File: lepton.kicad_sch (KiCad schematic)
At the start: 33 parts, among them U10 ME6216A28XG, U12 3N25000G33YC, U13 TD6810, U14 TD6810, U5 Flir_LEPTON

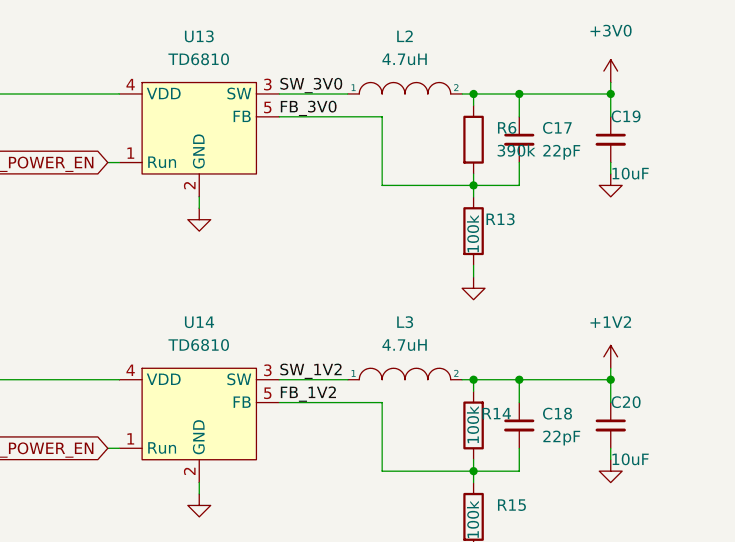
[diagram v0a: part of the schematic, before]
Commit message: Low power version WIP
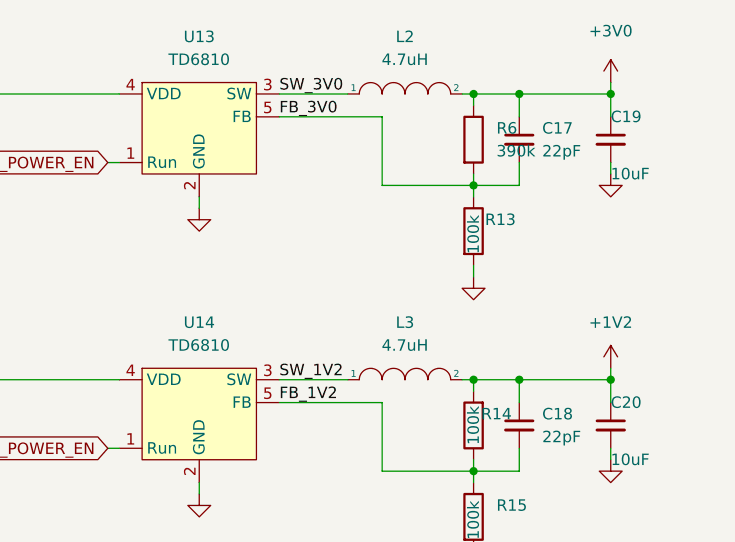
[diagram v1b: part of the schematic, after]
